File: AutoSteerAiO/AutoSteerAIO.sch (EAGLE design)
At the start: 88 parts, among them K4 CB1A-P-12V, U1 VX7805-1000

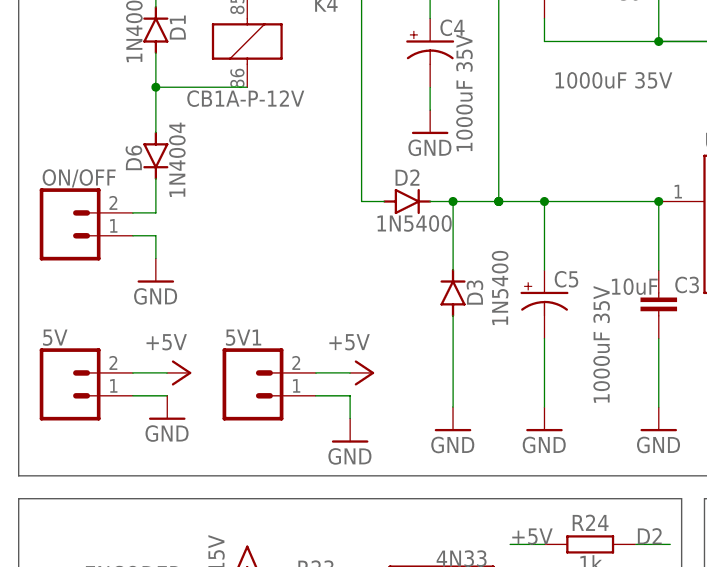
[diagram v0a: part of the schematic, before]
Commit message: Add files via upload
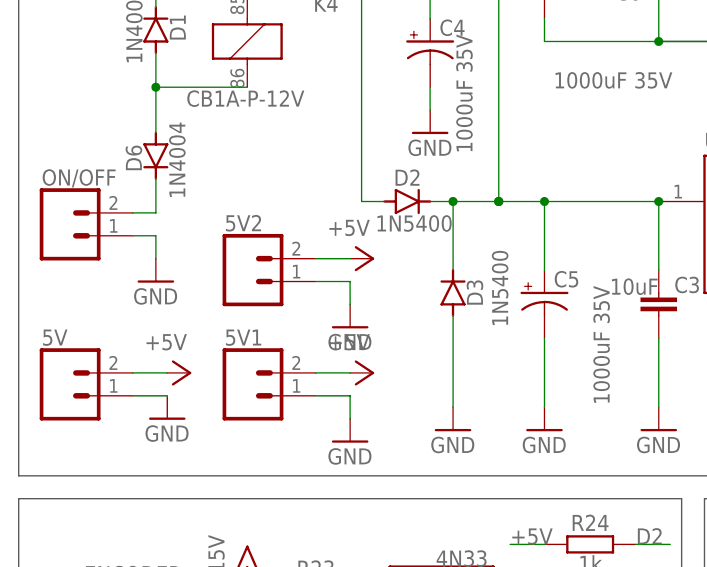
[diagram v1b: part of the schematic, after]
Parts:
- added 5V2: CONNECTOR 1x2 PINS, SparkFun-Connectors:CONN_02
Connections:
- net +5V: now also 5V2.2
- net GND: now also 5V2.1
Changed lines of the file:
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@@
 <part name="P+17" library="supply1" library_urn="urn:adsk.eagle:library:371" deviceset="+15V" device=""/>
 <part name="GND32" library="supply1" library_urn="urn:adsk.eagle:library:371" deviceset="GND" device=""/>
+<part name="5V2" library="SparkFun-Connectors" library_urn="urn:adsk.eagle:library:513" deviceset="CONN_02" device="" package3d_urn="urn:adsk.eagle:package:38039/1" value="CONNECTOR 1x2 PINS">
+<attribute name="MF" value=""/>
+<attribute name="MPN" value=""/>
+<attribute name="OC_NEWARK" value="unknown"/>
+</part>
+<part name="P+18" library="supply1" library_urn="urn:adsk.eagle:library:371" deviceset="+5V" device=""/>
+<part name="GND35" library="supply1" library_urn="urn:adsk.eagle:library:371" deviceset="GND" device=""/>
 </parts>
 <sheets>
@@
 <attribute name="VALUE" x="133.35" y="217.17" size="1.778" layer="96"/>
 </instance>
+<instance part="5V2" gate="G$1" x="7.62" y="222.25" smashed="yes">
+<attribute name="NAME" x="5.08" y="227.838" size="1.778" layer="95" font="vector"/>
+<attribute name="OC_NEWARK" x="7.62" y="222.25" size="1.778" layer="96" display="off"/>
+<attribute name="MF" x="7.62" y="222.25" size="1.778" layer="96" display="off"/>
+<attribute name="MPN" x="7.62" y="222.25" size="1.778" layer="96" display="off"/>
+</instance>
+<instance part="P+18" gate="1" x="21.59" y="224.79" smashed="yes" rot="R270">
+<attribute name="VALUE" x="16.51" y="227.33" size="1.778" layer="96"/>
+</instance>
+<instance part="GND35" gate="1" x="19.05" y="217.17" smashed="yes">
+<attribute name="VALUE" x="16.51" y="214.63" size="1.778" layer="96"/>
+</instance>
 </instances>
 <busses>
@@
 <pinref part="P+15" gate="1" pin="+5V"/>
 <wire x1="15.24" y1="212.09" x2="19.05" y2="212.09" width="0.1524" layer="91"/>
+</segment>
+<segment>
+<pinref part="5V2" gate="G$1" pin="2"/>
+<pinref part="P+18" gate="1" pin="+5V"/>
+<wire x1="15.24" y1="224.79" x2="19.05" y2="224.79" width="0.1524" layer="91"/>
 </segment>
 </net>
@@
 <wire x1="132.08" y1="222.25" x2="135.89" y2="222.25" width="0.1524" layer="91"/>
 </segment>
+<segment>
+<pinref part="GND35" gate="1" pin="GND"/>
+<pinref part="5V2" gate="G$1" pin="1"/>
+<wire x1="19.05" y1="219.71" x2="19.05" y2="222.25" width="0.1524" layer="91"/>
+<wire x1="19.05" y1="222.25" x2="15.24" y2="222.25" width="0.1524" layer="91"/>
+</segment>
 </net>
